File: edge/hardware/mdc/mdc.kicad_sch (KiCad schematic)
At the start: 8 parts

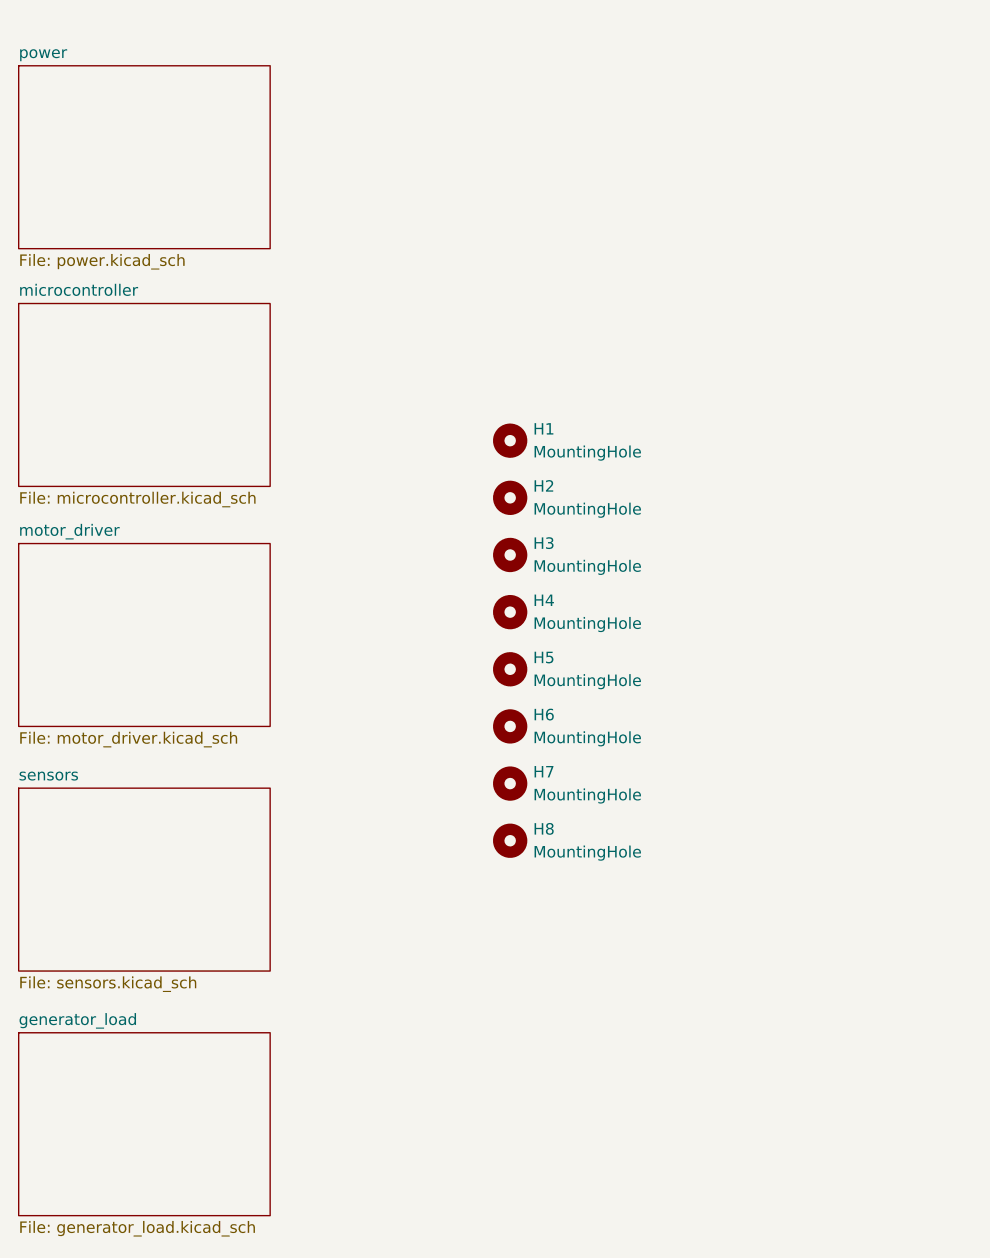
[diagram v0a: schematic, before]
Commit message: update rev3.0 schematic and layout
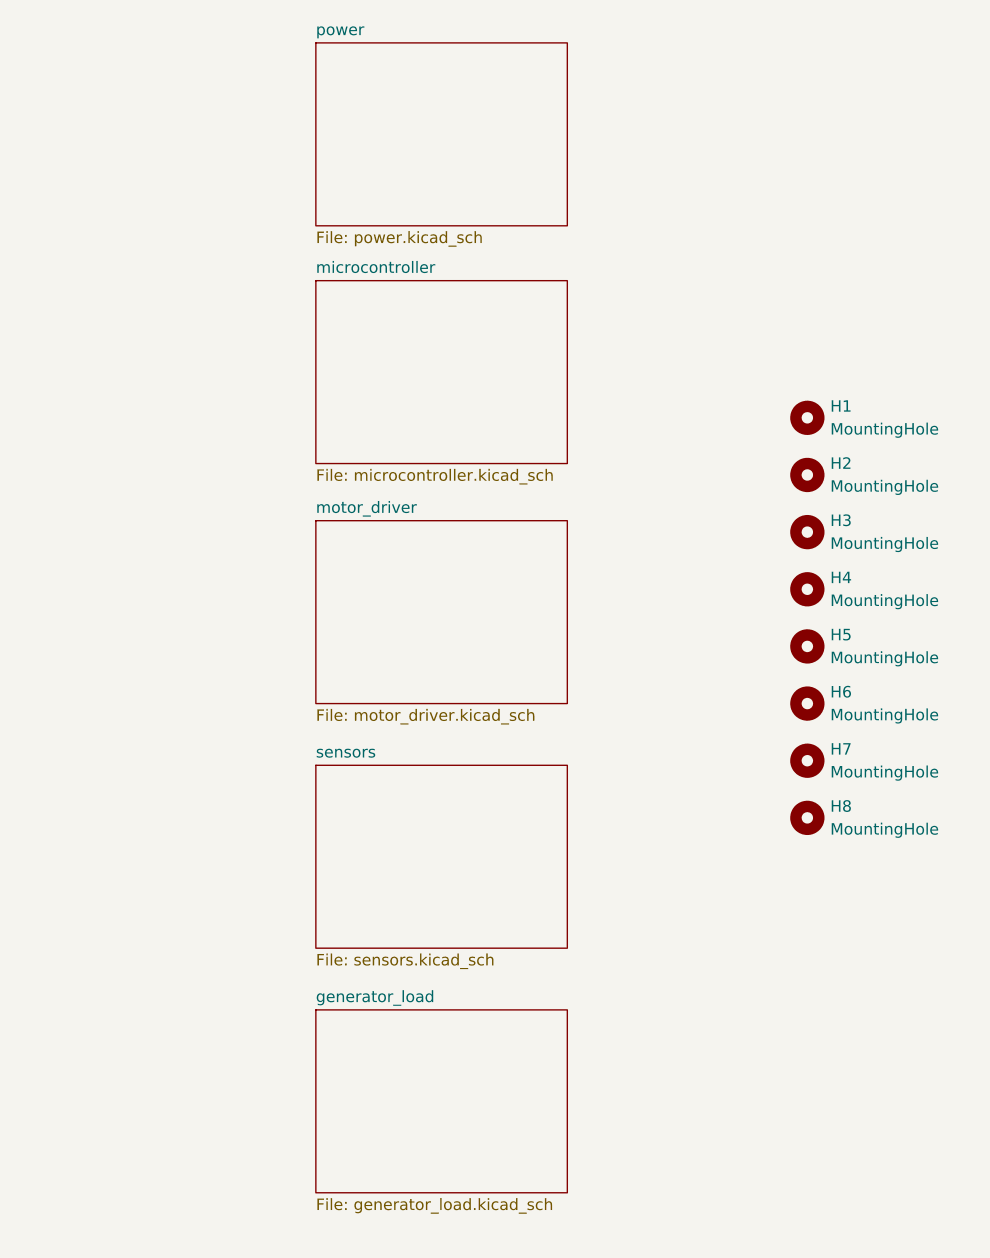
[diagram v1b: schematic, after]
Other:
- moved on the sheet: H1, H2, H3, H4, H5, H6, H7, H8
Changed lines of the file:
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@@
 	(title_block
 		(title "Motor Data Collector")
-		(date "2026-08-09")
+		(date "2026-08-10")
 		(rev "3.0")
 		(comment 1 "Department of EECS- AIoT and Energy Management Lab")
@@
 	(symbol
 		(lib_id "Mechanical:MountingHole")
-		(at 130.81 111.76 0)
+		(at 163.83 109.22 0)
 		(unit 1)
 		(body_style 1)
@@
 		(fields_autoplaced yes)
 		(property "Reference" "H6"
-			(at 133.35 110.4899 0)
+			(at 166.37 107.9499 0)
 			(show_name no)
 			(do_not_autoplace no)
@@
 		)
 		(property "Value" "MountingHole"
-			(at 133.35 113.0299 0)
+			(at 166.37 110.4899 0)
 			(show_name no)
 			(do_not_autoplace no)
@@
 		)
 		(property "Footprint" "MountingHole:MountingHole_3.2mm_M3"
-			(at 130.81 111.76 0)
+			(at 163.83 109.22 0)
 			(hide yes)
 			(show_name no)
@@
 		)
 		(property "Datasheet" ""
-			(at 130.81 111.76 0)
+			(at 163.83 109.22 0)
 			(hide yes)
 			(show_name no)
@@
 		)
 		(property "Description" "Mounting Hole without connection"
-			(at 130.81 111.76 0)
+			(at 163.83 109.22 0)
 			(hide yes)
 			(show_name no)
@@
 	(symbol
 		(lib_id "Mechanical:MountingHole")
-		(at 130.81 124.46 0)
+		(at 163.83 121.92 0)
 		(unit 1)
 		(body_style 1)
@@
 		(fields_autoplaced yes)
 		(property "Reference" "H8"
-			(at 133.35 123.1899 0)
+			(at 166.37 120.6499 0)
 			(show_name no)
 			(do_not_autoplace no)
@@
 		)
 		(property "Value" "MountingHole"
-			(at 133.35 125.7299 0)
+			(at 166.37 123.1899 0)
 			(show_name no)
 			(do_not_autoplace no)
@@
 		)
 		(property "Footprint" "MountingHole:MountingHole_3.2mm_M3"
-			(at 130.81 124.46 0)
+			(at 163.83 121.92 0)
 			(hide yes)
 			(show_name no)
@@
 		)
 		(property "Datasheet" ""
-			(at 130.81 124.46 0)
+			(at 163.83 121.92 0)
 			(hide yes)
 			(show_name no)
@@
 		)
 		(property "Description" "Mounting Hole without connection"
-			(at 130.81 124.46 0)
+			(at 163.83 121.92 0)
 			(hide yes)
 			(show_name no)
@@
 	(symbol
 		(lib_id "Mechanical:MountingHole")
-		(at 130.81 80.01 0)
+		(at 163.83 77.47 0)
 		(unit 1)
 		(body_style 1)
@@
 		(fields_autoplaced yes)
 		(property "Reference" "H1"
-			(at 133.35 78.7399 0)
+			(at 166.37 76.1999 0)
 			(show_name no)
 			(do_not_autoplace no)
@@
 		)
 		(property "Value" "MountingHole"
-			(at 133.35 81.2799 0)
+			(at 166.37 78.7399 0)
 			(show_name no)
 			(do_not_autoplace no)
@@
 		)
 		(property "Footprint" "MountingHole:MountingHole_4.3mm_M4"
-			(at 130.81 80.01 0)
+			(at 163.83 77.47 0)
 			(hide yes)
 			(show_name no)
@@
 		)
 		(property "Datasheet" ""
-			(at 130.81 80.01 0)
+			(at 163.83 77.47 0)
 			(hide yes)
 			(show_name no)
@@
 		)
 		(property "Description" "Mounting Hole without connection"
-			(at 130.81 80.01 0)
+			(at 163.83 77.47 0)
 			(hide yes)
 			(show_name no)
@@
 	(symbol
 		(lib_id "Mechanical:MountingHole")
-		(at 130.81 99.06 0)
+		(at 163.83 96.52 0)
 		(unit 1)
 		(body_style 1)
@@
 		(fields_autoplaced yes)
 		(property "Reference" "H4"
-			(at 133.35 97.7899 0)
+			(at 166.37 95.2499 0)
 			(show_name no)
 			(do_not_autoplace no)
@@
 		)
 		(property "Value" "MountingHole"
-			(at 133.35 100.3299 0)
+			(at 166.37 97.7899 0)
 			(show_name no)
 			(do_not_autoplace no)
@@
 		)
 		(property "Footprint" "MountingHole:MountingHole_4.3mm_M4"
-			(at 130.81 99.06 0)
+			(at 163.83 96.52 0)
 			(hide yes)
 			(show_name no)
@@
 		)
 		(property "Datasheet" ""
-			(at 130.81 99.06 0)
+			(at 163.83 96.52 0)
 			(hide yes)
 			(show_name no)
@@
 		)
 		(property "Description" "Mounting Hole without connection"
-			(at 130.81 99.06 0)
+			(at 163.83 96.52 0)
 			(hide yes)
 			(show_name no)
@@
 	(symbol
 		(lib_id "Mechanical:MountingHole")
-		(at 130.81 86.36 0)
+		(at 163.83 83.82 0)
 		(unit 1)
 		(body_style 1)
@@
 		(fields_autoplaced yes)
 		(property "Reference" "H2"
-			(at 133.35 85.0899 0)
+			(at 166.37 82.5499 0)
 			(show_name no)
 			(do_not_autoplace no)
@@
 		)
 		(property "Value" "MountingHole"
-			(at 133.35 87.6299 0)
+			(at 166.37 85.0899 0)
 			(show_name no)
 			(do_not_autoplace no)
@@
 		)
 		(property "Footprint" "MountingHole:MountingHole_4.3mm_M4"
-			(at 130.81 86.36 0)
+			(at 163.83 83.82 0)
 			(hide yes)
 			(show_name no)
@@
 		)
 		(property "Datasheet" ""
-			(at 130.81 86.36 0)
+			(at 163.83 83.82 0)
 			(hide yes)
 			(show_name no)
@@
 		)
 		(property "Description" "Mounting Hole without connection"
-			(at 130.81 86.36 0)
+			(at 163.83 83.82 0)
 			(hide yes)
 			(show_name no)
@@
 	(symbol
 		(lib_id "Mechanical:MountingHole")
-		(at 130.81 105.41 0)
+		(at 163.83 102.87 0)
 		(unit 1)
 		(body_style 1)
@@
 		(fields_autoplaced yes)
 		(property "Reference" "H5"
-			(at 133.35 104.1399 0)
+			(at 166.37 101.5999 0)
 			(show_name no)
 			(do_not_autoplace no)
@@
 		)
 		(property "Value" "MountingHole"
-			(at 133.35 106.6799 0)
+			(at 166.37 104.1399 0)
 			(show_name no)
 			(do_not_autoplace no)
@@
 		)
 		(property "Footprint" "MountingHole:MountingHole_3.2mm_M3"
-			(at 130.81 105.41 0)
+			(at 163.83 102.87 0)
 			(hide yes)
 			(show_name no)
@@
 		)
 		(property "Datasheet" ""
-			(at 130.81 105.41 0)
+			(at 163.83 102.87 0)
 			(hide yes)
 			(show_name no)
@@
 		)
 		(property "Description" "Mounting Hole without connection"
-			(at 130.81 105.41 0)
+			(at 163.83 102.87 0)
 			(hide yes)
 			(show_name no)
@@
 	(symbol
 		(lib_id "Mechanical:MountingHole")
-		(at 130.81 118.11 0)
+		(at 163.83 115.57 0)
 		(unit 1)
 		(body_style 1)
@@
 		(fields_autoplaced yes)
 		(property "Reference" "H7"
-			(at 133.35 116.8399 0)
+			(at 166.37 114.2999 0)
 			(show_name no)
 			(do_not_autoplace no)
@@
 		)
 		(property "Value" "MountingHole"
-			(at 133.35 119.3799 0)
+			(at 166.37 116.8399 0)
 			(show_name no)
 			(do_not_autoplace no)
@@
 		)
 		(property "Footprint" "MountingHole:MountingHole_3.2mm_M3"
-			(at 130.81 118.11 0)
+			(at 163.83 115.57 0)
 			(hide yes)
 			(show_name no)
@@
 		)
 		(property "Datasheet" ""
-			(at 130.81 118.11 0)
+			(at 163.83 115.57 0)
 			(hide yes)
 			(show_name no)
@@
 		)
 		(property "Description" "Mounting Hole without connection"
-			(at 130.81 118.11 0)
+			(at 163.83 115.57 0)
 			(hide yes)
 			(show_name no)
@@
 	(symbol
 		(lib_id "Mechanical:MountingHole")
-		(at 130.81 92.71 0)
+		(at 163.83 90.17 0)
 		(unit 1)
 		(body_style 1)
@@
 		(fields_autoplaced yes)
 		(property "Reference" "H3"
-			(at 133.35 91.4399 0)
+			(at 166.37 88.8999 0)
 			(show_name no)
 			(do_not_autoplace no)
@@
 		)
 		(property "Value" "MountingHole"
-			(at 133.35 93.9799 0)
+			(at 166.37 91.4399 0)
 			(show_name no)
 			(do_not_autoplace no)
@@
 		)
 		(property "Footprint" "MountingHole:MountingHole_4.3mm_M4"
-			(at 130.81 92.71 0)
+			(at 163.83 90.17 0)
 			(hide yes)
 			(show_name no)
@@
 		)
 		(property "Datasheet" ""
-			(at 130.81 92.71 0)
+			(at 163.83 90.17 0)
 			(hide yes)
 			(show_name no)
@@
 		)
 		(property "Description" "Mounting Hole without connection"
-			(at 130.81 92.71 0)
+			(at 163.83 90.17 0)
 			(hide yes)
 			(show_name no)
@@
 	)
 	(sheet
-		(at 76.2 64.77)
+		(at 109.22 62.23)
 		(size 27.94 20.32)
 		(exclude_from_sim no)
@@
 		)
 		(property "Sheetname" "microcontroller"
-			(at 76.2 64.0584 0)
+			(at 109.22 61.5184 0)
 			(show_name no)
 			(do_not_autoplace no)
@@
 		)
 		(property "Sheetfile" "microcontroller.kicad_sch"
-			(at 76.2 85.6746 0)
+			(at 109.22 83.1346 0)
 			(show_name no)
 			(do_not_autoplace no)
@@
 	)
 	(sheet
-		(at 76.2 38.354)
+		(at 109.22 35.814)
 		(size 27.94 20.32)
 		(exclude_from_sim no)
@@
 		)
 		(property "Sheetname" "power"
-			(at 76.2 37.6424 0)
+			(at 109.22 35.1024 0)
 			(show_name no)
 			(do_not_autoplace no)
@@
 		)
 		(property "Sheetfile" "power.kicad_sch"
-			(at 76.2 59.2586 0)
+			(at 109.22 56.7186 0)
 			(show_name no)
 			(do_not_autoplace no)
@@
 	)
 	(sheet
-		(at 76.2 145.796)
+		(at 109.22 143.256)
 		(size 27.94 20.32)
 		(exclude_from_sim no)
@@
 		)
 		(property "Sheetname" "generator_load"
-			(at 76.2 145.0844 0)
+			(at 109.22 142.5444 0)
 			(show_name no)
 			(do_not_autoplace no)
@@
 		)
 		(property "Sheetfile" "generator_load.kicad_sch"
-			(at 76.2 166.7006 0)
+			(at 109.22 164.1606 0)
 			(show_name no)
 			(do_not_autoplace no)
@@
 	)
 	(sheet
-		(at 76.2 91.44)
+		(at 109.22 88.9)
 		(size 27.94 20.32)
 		(exclude_from_sim no)
@@
 		)
 		(property "Sheetname" "motor_driver"
-			(at 76.2 90.7284 0)
+			(at 109.22 88.1884 0)
 			(show_name no)
 			(do_not_autoplace no)
@@
 		)
 		(property "Sheetfile" "motor_driver.kicad_sch"
-			(at 76.2 112.3446 0)
+			(at 109.22 109.8046 0)
 			(show_name no)
 			(do_not_autoplace no)
@@
 	)
 	(sheet
-		(at 76.2 118.618)
+		(at 109.22 116.078)
 		(size 27.94 20.32)
 		(exclude_from_sim no)
@@
 		)
 		(property "Sheetname" "sensors"
-			(at 76.2 117.9064 0)
+			(at 109.22 115.3664 0)
 			(show_name no)
 			(do_not_autoplace no)
@@
 		)
 		(property "Sheetfile" "sensors.kicad_sch"
-			(at 76.2 139.5226 0)
-			(show_name no)
-			(do_not_autoplace no)
+			(at 109.22 136.9826 0)
+			(show_name no)
+			(do_not_autoplace no)
